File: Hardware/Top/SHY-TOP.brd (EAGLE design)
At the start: 160 x 100 mm, 0 parts

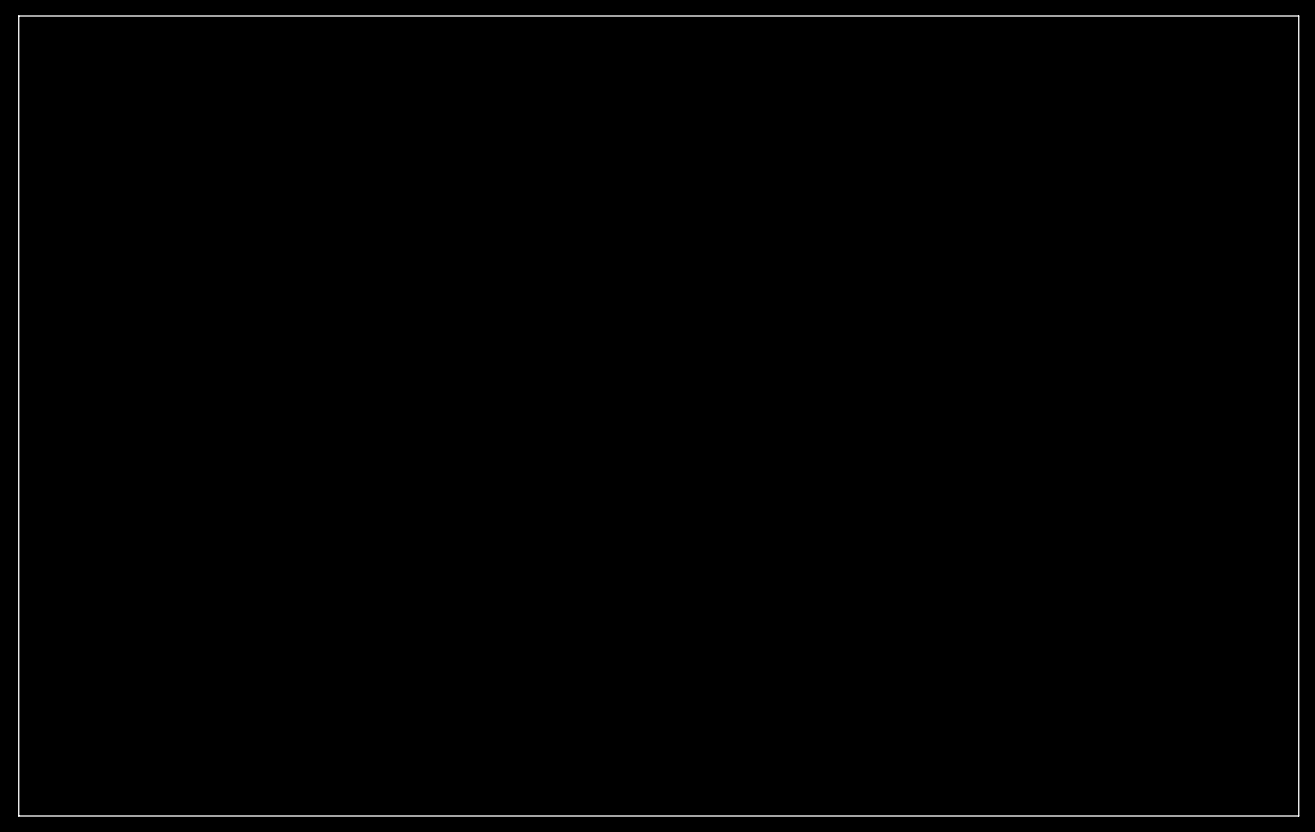
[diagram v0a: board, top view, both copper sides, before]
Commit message: Add top board
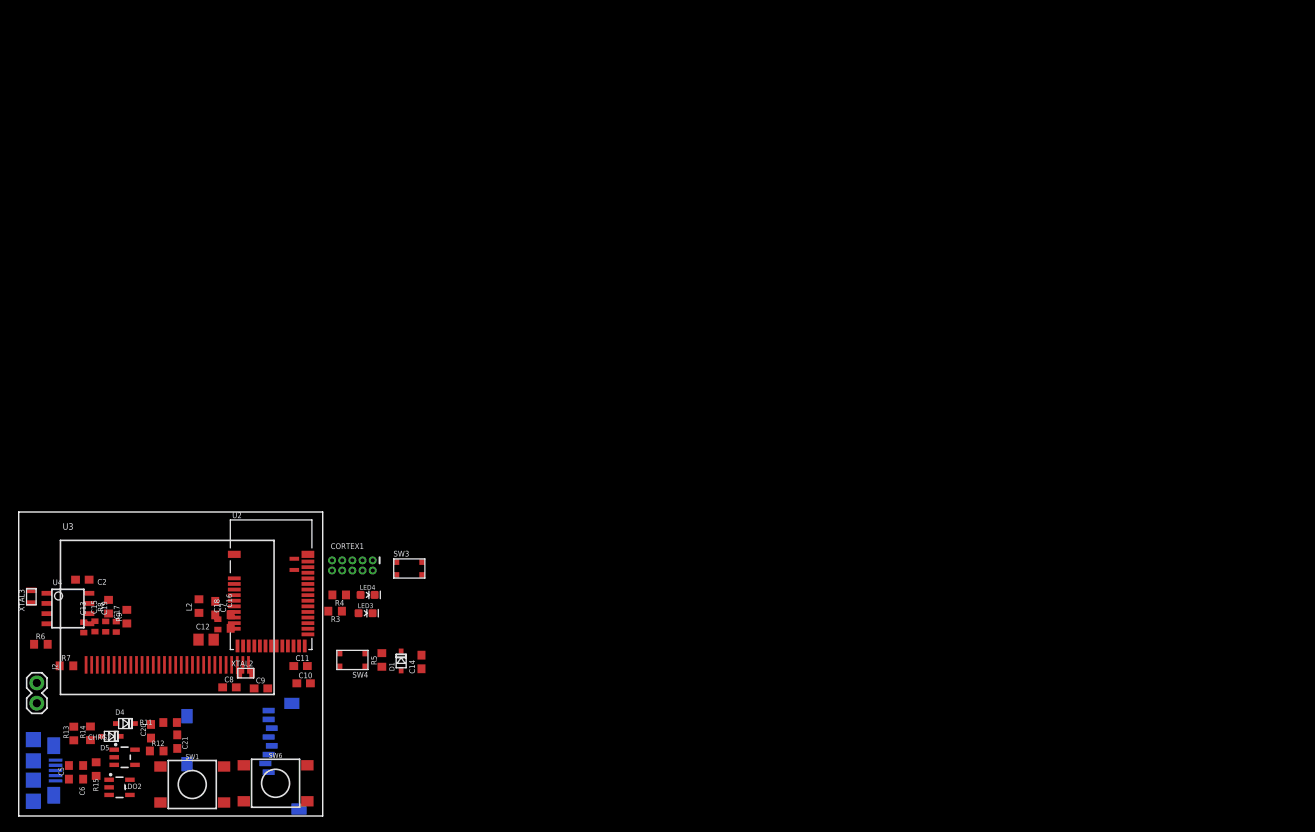
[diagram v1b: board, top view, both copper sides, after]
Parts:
- added C10, C11: 300p, LinnesLab-Passives:C0603
- added C12: 10u, LinnesLab-Passives:C0805
- added C13, C15, C17, C18, C19: 2.2uF, LinnesLab-Passives:C0402
- added C14: 100n, LinnesLab-Passives:C0603
- added C16: 10uF, LinnesLab-Passives:C0603
- added C2, C5, C6, C7: 1u, LinnesLab-Passives:C0603
- added C20, C21: 4.7u, LinnesLab-Passives:C0603
- added C8, C9: (no value), LinnesLab-Passives:C0603
- added CHRG2: MCP73831, LinnesLab-Power:SOT23-5
- added CORTEX1: CORTEX_DEBUG_PTH, LinnesLab-Connectors:2X5-PTH-1.27MM
- added D1, D4, D5: (no value), LinnesLab-DiscreteSemi:USC
- added J2: (no value), LinnesLab-Connectors:1X02
- added L2: 10u, LinnesLab-Passives:L0603
- added LDO2: MIC5504, LinnesLab-Power:SOT23-5
- added LED3: RED, LinnesLab-LED:LED-0603
- added LED4: BLUE, LinnesLab-LED:LED-0603
- added R11: (no value), LinnesLab-Passives:R0603
- added R12, R13, R14, R15: 100k, LinnesLab-Passives:R0603
- added R3, R4: 1k, LinnesLab-Passives:R0603
- added R5, R6, R8, R9: 10k, LinnesLab-Passives:R0603
- added R7: 390k, LinnesLab-Passives:R0603
- added SD2: (no value), LinnesLab-Connectors:MICROSD
- added SW1, SW6: SWITCH.MOM, LinnesLab-Switches:TACTILE_SWITCH_SMD_6.2MM_TALL
- added SW3, SW4: (no value), LinnesLab-Switches:BUTTON-GULLWING
- added U2: NRF52832_MODULE_MDBT42, LinnesLab-Microcontrollers:BLE_MODULE_RAYTAC_MDBT42
- added U3: (no value), LinnesLab-Displays:UG-2864HSWEG01_0.96IN_NO-WRAPAROUND
- added U4: PCF8523, LinnesLab-Clocks:SO8
- added USB2: USB.MICRO-BIGGERPADS, LinnesLab-Connectors:USB-MICRO-01.BIGGERPADS
- added XTAL2: 32.768kHz, LinnesLab-Clocks:2-SMD.NOLEAD.2.0MMTO1.2MM
- added XTAL3: 32.7680kHz, LinnesLab-Clocks:2-SMD.NOLEAD.2.0MMTO1.2MM
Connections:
- new net 3.3V: C12.2, C17.2, C19.2, C2.1, C6.1, CORTEX1.1, D1.-, LDO2.5, R15.2, R5.2, R8.2, R9.2, SD2.4, U2.11, U3.6, U3.9, U4.8
- new net BATT: R13.1, R14.2
- new net CD1: SD2.CD1
- new net CD2: SD2.CD2
- new net CHRG.STAT: CHRG2.1, R12.1
- new net CS.OLED: U3.13
- new net DC.OLED: U3.15
- new net DFU: SW3.3, U2.34
- new net DTR: C14.1
- new net FRST: U2.38
- new net GND: C10.2, C11.2, C12.1, C16.1, C17.1, C18.1, C19.1, C2.2, C20.2, C21.1, C5.1, C6.2, C7.2, C8.1, C9.2, CHRG2.2, CORTEX1.3, CORTEX1.5, CORTEX1.7, CORTEX1.9, J2.1, LDO2.2, LED3.C, LED4.C, R11.1, R14.1, R15.1, R6.1, R7.2, SD2.6, SD2.MT1, SD2.MT2, SW1.B1, SW1.B2, SW3.1, SW4.3, SW6.B1, SW6.B2, U2.1, U2.12, U2.24, U2.39, U3.1, U3.10, U3.12, U3.29, U3.30, U3.8, U4.4, USB2.5
- new net LED1: R3.2, U2.31
- new net LED2: R4.2, U2.33
- new net MISO: SD2.7, U2.28
- new net MOSI: SD2.3, U2.27, U3.19
- new net N$1: R6.2, U3.11
- new net N$10: LED4.A, R4.1
- new net N$11: L2.1, U2.10
- new net N$12: C7.1, L2.2, U2.9
- new net N$13: C16.2, U3.28
- new net N$14: CORTEX1.8
- new net N$15: C18.2, U3.27
- new net N$17: CHRG2.5, R11.2
- new net N$19: U4.2, XTAL3.P$1
- new net N$2: R7.1, U3.26
- new net N$20: U4.1, XTAL3.P$2
- new net N$3: C13.2, U3.2
- new net N$4: C8.2, U2.13, XTAL2.P$1
- new net N$5: C13.1, U3.3
- new net N$6: C9.1, U2.14, XTAL2.P$2
- new net N$7: C15.2, U3.4
- new net N$8: C15.1, U3.5
- new net N$9: LED3.A, R3.1
- new net P0.09/NFC1: C11.1, U2.22
- new net P0.10/NFC2: C10.1, U2.23
- new net RESET: C14.2, CORTEX1.10, D1.+, R5.1, SW4.1, U2.35
- new net RESET.OLED: U3.14
- new net RXD: U2.21
- new net SCK: SD2.5, U2.26, U3.18
- new net SCL: R8.1, U2.3, U4.6
- new net SD.CS: SD2.2
- new net SDA: R9.1, U2.2, U4.5
- new net SW1: SW1.A1, SW6.A1
- new net SWCLK: CORTEX1.4, U2.36
- new net SWDIO: CORTEX1.2, U2.37
- new net SWO: CORTEX1.6, U2.32
- new net TXD: U2.19
- new net USB+: USB2.3
- new net USB-: USB2.2
- new net VBAT: U4.3
- new net VIN: C21.2, C5.2, CHRG2.4, D4.-, D5.-, LDO2.1, LDO2.3, R12.2
- new net VLIPO: C20.1, CHRG2.3, D4.+, J2.2, R13.2
- new net V_USB: D5.+, USB2.1
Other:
- board size 160 x 100 mm -> 38 x 38 mm
